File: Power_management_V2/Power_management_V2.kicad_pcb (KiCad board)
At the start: 4 copper layers, 76.5 x 63 mm, 56 parts, among them J1 640388-3, U1 SIC43x, U2 SIC43x, U3 TPS3711DDCR

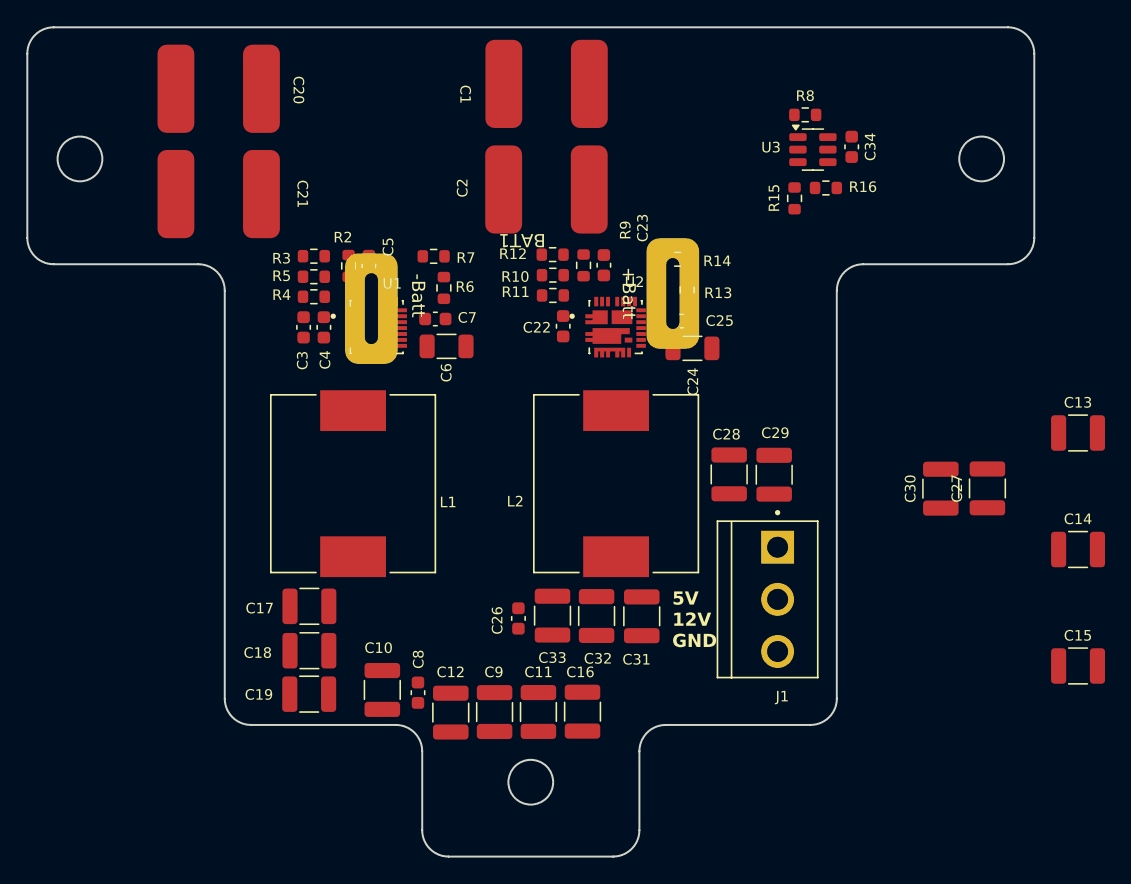
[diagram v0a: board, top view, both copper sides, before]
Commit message: Hoan thien Sap xep Linh kien
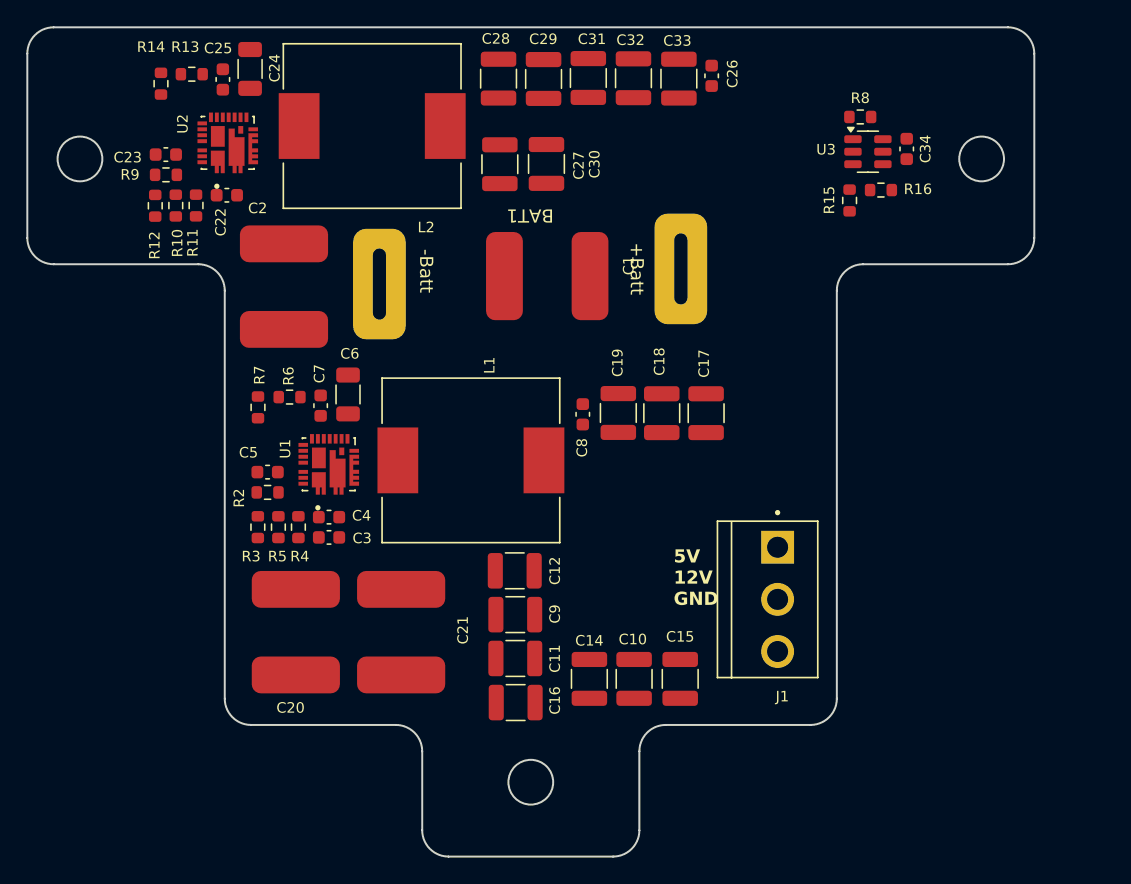
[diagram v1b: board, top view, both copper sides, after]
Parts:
- removed C13: 22u/25V/1210, Capacitor_SMD:C_1210_3225Metric
- moved C27 44.5 mm to (118.0, 65.1), turned to -90 degrees
- moved C26 43.8 mm to (134.0, 58.4), turned to -90 degrees
- moved C33 41.9 mm to (131.6, 58.6), turned to 90 degrees
- moved C20 41.7 mm to (102.5, 100.6), turned to -90 degrees
- moved R14 41.5 mm to (92.2, 59.0), turned to -90 degrees
- moved C31 41.1 mm to (124.7, 58.5), turned to 90 degrees
- moved R13 41.1 mm to (94.5, 58.3), turned to 180 degrees
- moved C32 41.0 mm to (128.1, 58.6), turned to 90 degrees
- moved C24 39.7 mm to (99.0, 57.9), turned to 90 degrees
- moved C25 39.4 mm to (96.9, 58.7), turned to 90 degrees
- moved C30 38.8 mm to (121.5, 65.1), turned to -90 degrees
- moved C14 38.4 mm to (124.8, 104.2), turned to -90 degrees
- moved C21 36.1 mm to (110.5, 100.6), turned to -90 degrees
- moved C28 34.8 mm to (117.9, 58.6)
- moved C29 34.8 mm to (121.3, 58.6)
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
